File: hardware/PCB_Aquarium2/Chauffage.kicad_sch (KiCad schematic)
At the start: 2 parts, among them J38 Conn_01x03

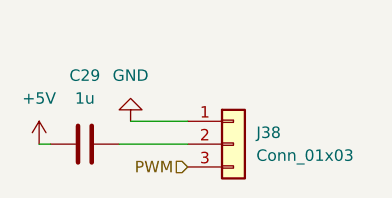
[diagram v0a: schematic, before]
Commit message: PCBs v4
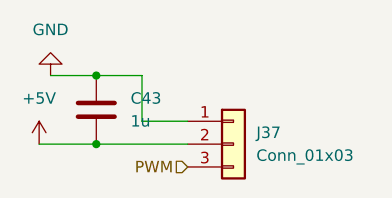
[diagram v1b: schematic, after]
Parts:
- renumbered C29 to C43, J38 to J37
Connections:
- net +5V: now also J37.2 (Pin_2)
- net GND: now also C43.2
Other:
- moved on the sheet: C43
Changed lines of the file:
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@@
 	(generator_version "9.0")
 	(paper "A4")
-	(wire
-		(pts
-			(xy 130.81 77.47) (xy 137.16 77.47)
-		)
-		(stroke
-			(width 0)
-			(type default)
-		)
-	)
-	(wire
-		(pts
-			(xy 129.54 80.01) (xy 137.16 80.01)
-		)
-		(stroke
-			(width 0)
-			(type default)
-		)
-	)
-	(wire
-		(pts
-			(xy 120.65 80.01) (xy 121.92 80.01)
+	(junction
+		(at 127 72.39)
+		(diameter 0)
+		(color 0 0 0 0)
+	)
+	(junction
+		(at 127 80.01)
+		(diameter 0)
+		(color 0 0 0 0)
+	)
+	(wire
+		(pts
+			(xy 121.92 72.39) (xy 127 72.39)
+		)
+		(stroke
+			(width 0)
+			(type default)
+		)
+	)
+	(wire
+		(pts
+			(xy 132.08 77.47) (xy 137.16 77.47)
+		)
+		(stroke
+			(width 0)
+			(type default)
+		)
+	)
+	(wire
+		(pts
+			(xy 127 80.01) (xy 137.16 80.01)
+		)
+		(stroke
+			(width 0)
+			(type default)
+		)
+	)
+	(wire
+		(pts
+			(xy 127 72.39) (xy 132.08 72.39)
+		)
+		(stroke
+			(width 0)
+			(type default)
+		)
+	)
+	(wire
+		(pts
+			(xy 132.08 72.39) (xy 132.08 77.47)
+		)
+		(stroke
+			(width 0)
+			(type default)
+		)
+	)
+	(wire
+		(pts
+			(xy 120.65 80.01) (xy 127 80.01)
 		)
 		(stroke
@@
 	(symbol
 		(lib_id "power:GND")
-		(at 130.81 77.47 180)
+		(at 121.92 72.39 180)
 		(unit 1)
 		(exclude_from_sim no)
@@
 		(dnp no)
 		(fields_autoplaced yes)
-		(property "Reference" "#PWR091"
-			(at 130.81 71.12 0)
+		(property "Reference" "#PWR089"
+			(at 121.92 66.04 0)
 			(effects
 				(font
@@
 		)
 		(property "Value" "GND"
-			(at 130.81 72.39 0)
+			(at 121.92 67.31 0)
 			(effects
 				(font
@@
 		)
 		(property "Footprint" ""
-			(at 130.81 77.47 0)
+			(at 121.92 72.39 0)
 			(effects
 				(font
@@
 		)
 		(property "Datasheet" ""
-			(at 130.81 77.47 0)
+			(at 121.92 72.39 0)
 			(effects
 				(font
@@
 		)
 		(property "Description" "Power symbol creates a global label with name \"GND\" , ground"
-			(at 130.81 77.47 0)
+			(at 121.92 72.39 0)
 			(effects
 				(font
@@
 			(project ""
 				(path "/4f9429d5-fbb3-48e9-90dd-7ff0c2950e6f/6996448a-079a-4fbd-aac0-272391141173"
-					(reference "#PWR091")
+					(reference "#PWR089")
 					(unit 1)
 				)
@@
 		(dnp no)
 		(fields_autoplaced yes)
-		(property "Reference" "J38"
+		(property "Reference" "J37"
 			(at 144.78 78.7399 0)
 			(effects
@@
 			(project "PCB_Aquarium2"
 				(path "/4f9429d5-fbb3-48e9-90dd-7ff0c2950e6f/6996448a-079a-4fbd-aac0-272391141173"
-					(reference "J38")
+					(reference "J37")
 					(unit 1)
 				)
@@
 	(symbol
 		(lib_id "Device:C")
-		(at 125.73 80.01 90)
+		(at 127 76.2 180)
 		(unit 1)
 		(exclude_from_sim no)
@@
 		(dnp no)
 		(fields_autoplaced yes)
-		(property "Reference" "C29"
-			(at 125.73 72.39 90)
-			(effects
-				(font
-					(size 1.27 1.27)
-				)
+		(property "Reference" "C43"
+			(at 130.81 74.9299 0)
+			(effects
+				(font
+					(size 1.27 1.27)
+				)
+				(justify right)
 			)
 		)
 		(property "Value" "1u"
-			(at 125.73 74.93 90)
-			(effects
-				(font
-					(size 1.27 1.27)
-				)
+			(at 130.81 77.4699 0)
+			(effects
+				(font
+					(size 1.27 1.27)
+				)
+				(justify right)
 			)
 		)
 		(property "Footprint" "Capacitor_SMD:C_0603_1608Metric"
-			(at 129.54 79.0448 0)
+			(at 126.0348 72.39 0)
 			(effects
 				(font
@@
 		)
 		(property "Datasheet" "~"
-			(at 125.73 80.01 0)
+			(at 127 76.2 0)
 			(effects
 				(font
@@
 		)
 		(property "Description" "Unpolarized capacitor"
-			(at 125.73 80.01 0)
+			(at 127 76.2 0)
 			(effects
 				(font
@@
 		)
 		(instances
-			(project ""
+			(project "PCB_Aquarium2"
 				(path "/4f9429d5-fbb3-48e9-90dd-7ff0c2950e6f/6996448a-079a-4fbd-aac0-272391141173"
-					(reference "C29")
+					(reference "C43")
 					(unit 1)
 				)
@@
 		(dnp no)
 		(fields_autoplaced yes)
-		(property "Reference" "#PWR090"
+		(property "Reference" "#PWR088"
 			(at 120.65 83.82 0)
 			(effects
@@
 			(project "PCB_Aquarium2"
 				(path "/4f9429d5-fbb3-48e9-90dd-7ff0c2950e6f/6996448a-079a-4fbd-aac0-272391141173"
-					(reference "#PWR090")
+					(reference "#PWR088")
 					(unit 1)
 				)
